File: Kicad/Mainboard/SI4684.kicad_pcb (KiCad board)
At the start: 2 copper layers, 100 x 68 mm, 91 parts, among them J1 DC IN, J2 Ant, J3 Headphones, J4 FRONT-PCB, J5 AUDIO, U1 MIC5504-1.8YM5, U2 LM2596T-5, U3 SI4684-A10-GM, U4 LM1117T-3.3, U5 TPA6130A2RTJTG4, U6 NE5532, X1 19.2MHz

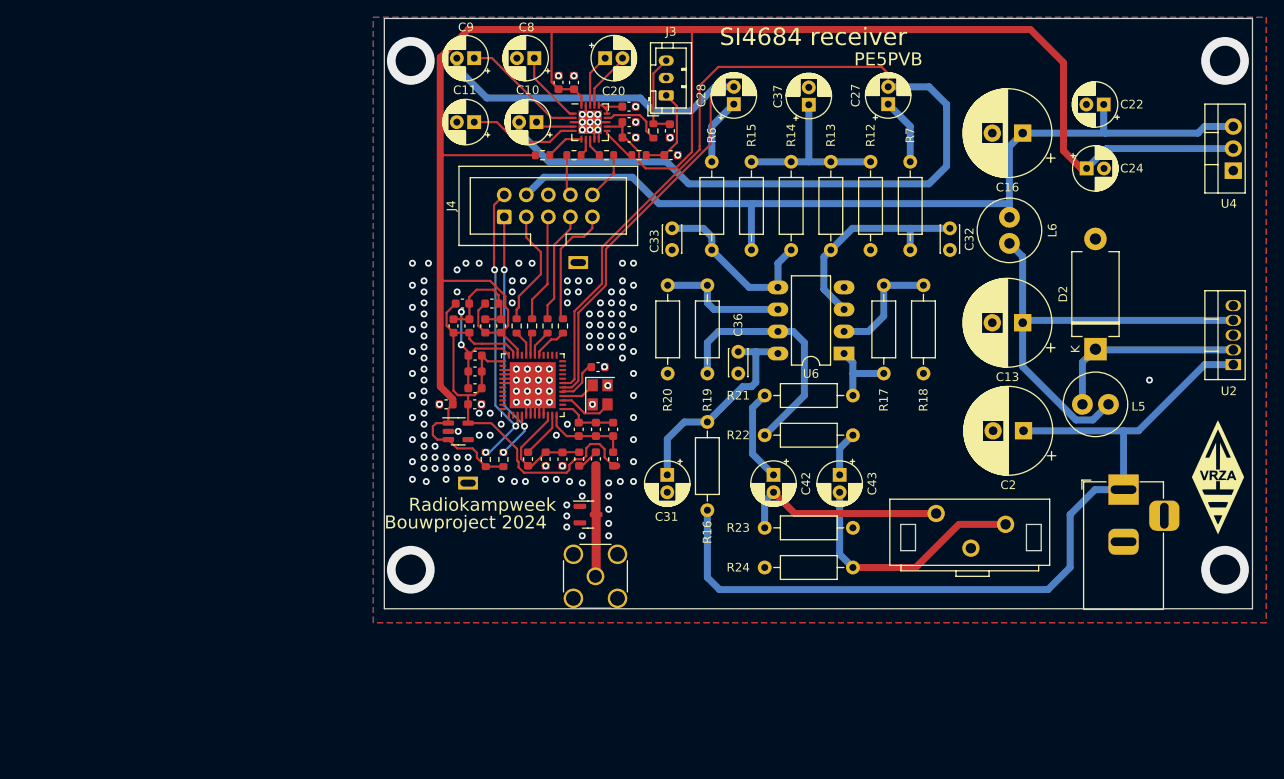
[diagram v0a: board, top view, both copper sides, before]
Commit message: Add files via upload
work in progress. not finished
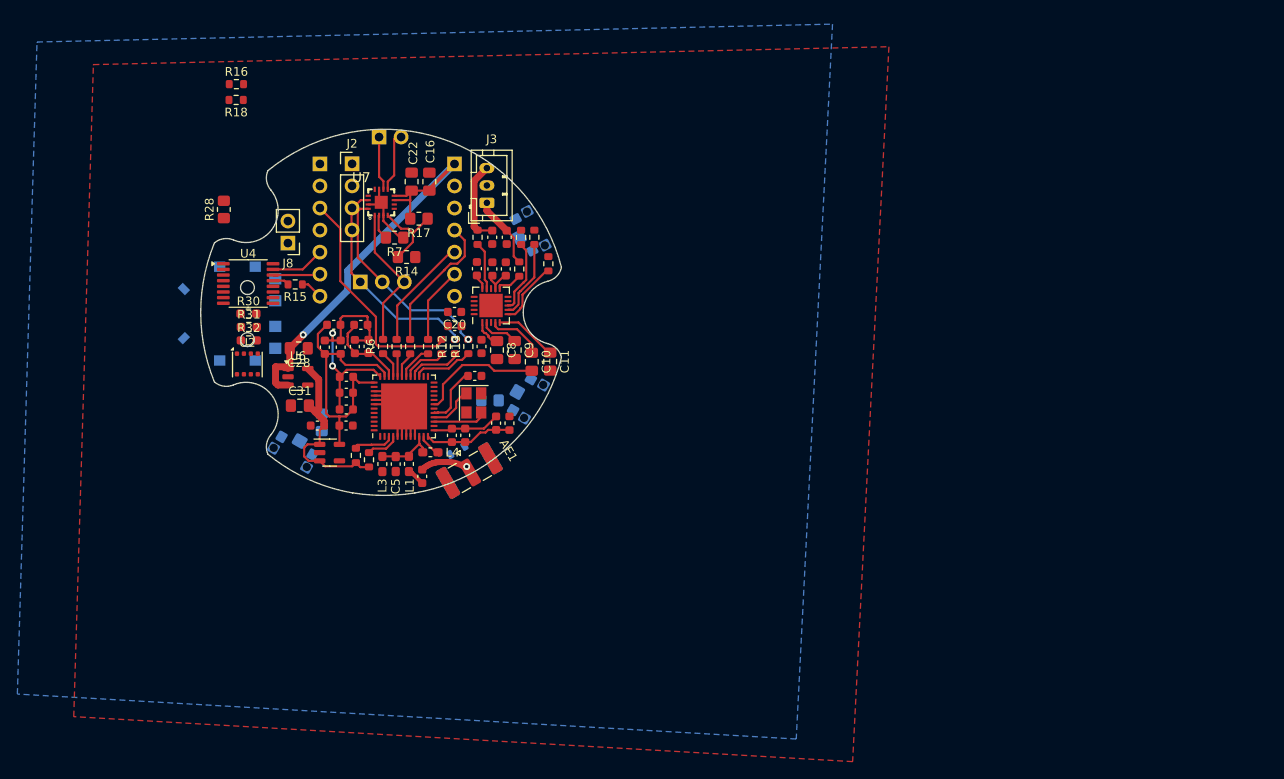
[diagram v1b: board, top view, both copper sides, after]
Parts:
- removed C13, C2: 220uF, Capacitor_THT:CP_Radial_D10.0mm_P3.50mm
- removed C24, C27, C37: 10uF, Capacitor_THT:CP_Radial_D5.0mm_P2.00mm
- removed C32, C33, C36: 10p, Capacitor_THT:C_Disc_D3.0mm_W2.0mm_P2.50mm
- removed C42, C43: 47uF, Capacitor_THT:CP_Radial_D5.0mm_P2.00mm
- removed D2: 1N5822, Diode_THT:D_DO-201_P12.70mm_Horizontal
- removed G***: LOGO, Library:VRZA
- removed J4: FRONT-PCB, Connector_IDC:IDC-Header_2x05_P2.54mm_Vertical
- removed L5: 33uH, Inductor_THT:L_Radial_D7.2mm_P3.00mm_Murata_1700
- removed L6: 22uH, Inductor_THT:L_Radial_D7.2mm_P3.00mm_Murata_1700
- removed R19: 4k7, Resistor_THT:R_Axial_DIN0207_L6.3mm_D2.5mm_P10.16mm_Horizontal
- removed R20: 3k9, Resistor_THT:R_Axial_DIN0207_L6.3mm_D2.5mm_P10.16mm_Horizontal
- removed R21, R22: 220, Resistor_THT:R_Axial_DIN0207_L6.3mm_D2.5mm_P10.16mm_Horizontal
- removed R23, R24: 100k, Resistor_THT:R_Axial_DIN0207_L6.3mm_D2.5mm_P10.16mm_Horizontal
- removed REF**: 25x25 can, Library:25x25 can
- added AE1: Antenna_Shield, Connector_Coaxial:SMA_Samtec_SMA-J-P-H-ST-EM1_EdgeMount, F.Cu at (109.5, 118.6)
- added J6: DISP RIGHT, Connector_PinHeader_2.54mm:PinHeader_1x07_P2.54mm_Vertical, B.Cu at (107.6, 83.0)
- added J7: Conn_01x02_Pin, Connector_PinHeader_2.54mm:PinHeader_1x02_P2.54mm_Vertical, B.Cu at (99.0, 80.0)
- added J8: Conn_01x02_Pin, Connector_PinHeader_2.54mm:PinHeader_1x02_P2.54mm_Vertical, F.Cu at (88.5, 92.2)
- added R27: 10k, Resistor_SMD:R_0805_2012Metric_Pad1.20x1.40mm_HandSolder, B.Cu at (92.4, 112.8)
- added R28: 10k, Resistor_SMD:R_0805_2012Metric_Pad1.20x1.40mm_HandSolder, F.Cu at (81.1, 88.3)
- added R29: 10k, Resistor_SMD:R_0805_2012Metric_Pad1.20x1.40mm_HandSolder, B.Cu at (111.7, 110.3)
- added R30: 10k, Resistor_SMD:R_0603_1608Metric_Pad0.98x0.95mm_HandSolder, F.Cu at (83.9, 100.3)
- added R31: 10k, Resistor_SMD:R_0603_1608Metric_Pad0.98x0.95mm_HandSolder, F.Cu at (84.0, 101.8)
- added R32: 10k, Resistor_SMD:R_0603_1608Metric_Pad0.98x0.95mm_HandSolder, F.Cu at (84.0, 103.4)
- added SW4: SW_Push, tp4056:SW_SPST_CK_KMS2xxGP, B.Cu at (89.1, 116.2)
- added SW5: SW_Push, tp4056:SW_SPST_CK_KMS2xxGP, B.Cu at (116.4, 90.8)
- added SW6: SW_Push, tp4056:SW_SPST_CK_KMS2xxGP, B.Cu at (116.1, 110.0)
- added U12: SIQ-02FVS3, tp4056:SW-SMD_SIQ-02FVS3_1, B.Cu at (81.7, 100.3)
- added U7: ~, tp4056:TQFN-16_L3.0-W3.0-P0.50-BL-EP1.5, F.Cu at (99.2, 87.5)
- C10, C28, C31, C9: value 10uF -> 1uF; footprint Capacitor_THT:CP_Radial_D5.0mm_P2.00mm -> Capacitor_SMD:C_0805_2012Metric_Pad1.18x1.45mm_HandSolder
- C11, C8: footprint Capacitor_THT:CP_Radial_D5.0mm_P2.00mm -> Capacitor_SMD:C_0805_2012Metric_Pad1.18x1.45mm_HandSolder
- C16: value 100uF -> 10uF; footprint Capacitor_THT:CP_Radial_D10.0mm_P3.50mm -> Capacitor_SMD:C_0805_2012Metric_Pad1.18x1.45mm_HandSolder
- C20: footprint Capacitor_THT:CP_Radial_D5.0mm_P2.00mm -> Capacitor_SMD:C_0603_1608Metric
- C22: value 10uF -> 100nF; footprint Capacitor_THT:CP_Radial_D5.0mm_P2.00mm -> Capacitor_SMD:C_0805_2012Metric_Pad1.18x1.45mm_HandSolder
- C5: footprint Capacitor_SMD:C_0603_1608Metric -> Capacitor_SMD:C_0603_1608Metric_Pad1.08x0.95mm_HandSolder
- D1: footprint Package_TO_SOT_SMD:SOT-23 -> Package_TO_SOT_SMD:SOT-23W; moved to B.Cu
- J1: value DC IN -> Conn_01x03; footprint Connector_BarrelJack:BarrelJack_Horizontal -> Connector_PinHeader_2.54mm:PinHeader_1x03_P2.54mm_Vertical; moved to B.Cu
- J2: value Ant -> Conn_01x04_Pin; footprint Connector_Coaxial:SMA_Amphenol_132134-16_Vertical -> Connector_PinHeader_2.54mm:PinHeader_1x04_P2.54mm_Vertical
- J5: value AUDIO -> DISP LEFT; footprint Library:FC68405_cinch -> Connector_PinHeader_2.54mm:PinHeader_1x07_P2.54mm_Vertical; moved to B.Cu
- L1, L3, L4: footprint Inductor_SMD:L_0603_1608Metric -> Inductor_SMD:L_0603_1608Metric_Pad1.05x0.95mm_HandSolder
- R12: value 39k -> 2k; footprint Resistor_THT:R_Axial_DIN0207_L6.3mm_D2.5mm_P10.16mm_Horizontal -> Resistor_SMD:R_0603_1608Metric
- R13: value 100k -> 2k; footprint Resistor_THT:R_Axial_DIN0207_L6.3mm_D2.5mm_P10.16mm_Horizontal -> Resistor_SMD:R_0603_1608Metric
- R14: value 100k -> 3k; footprint Resistor_THT:R_Axial_DIN0207_L6.3mm_D2.5mm_P10.16mm_Horizontal -> Resistor_SMD:R_0805_2012Metric_Pad1.20x1.40mm_HandSolder
- R15: value 39k -> 100; footprint Resistor_THT:R_Axial_DIN0207_L6.3mm_D2.5mm_P10.16mm_Horizontal -> Resistor_SMD:R_0603_1608Metric
- R16: value 10 -> 0; footprint Resistor_THT:R_Axial_DIN0207_L6.3mm_D2.5mm_P10.16mm_Horizontal -> Resistor_SMD:R_0603_1608Metric
- R17: value 4k7 -> 680K; footprint Resistor_THT:R_Axial_DIN0207_L6.3mm_D2.5mm_P10.16mm_Horizontal -> Resistor_SMD:R_0805_2012Metric_Pad1.20x1.40mm_HandSolder
- R18: value 3k9 -> 0; footprint Resistor_THT:R_Axial_DIN0207_L6.3mm_D2.5mm_P10.16mm_Horizontal -> Resistor_SMD:R_0603_1608Metric
- R6: value 4k7 -> 600; footprint Resistor_THT:R_Axial_DIN0207_L6.3mm_D2.5mm_P10.16mm_Horizontal -> Resistor_SMD:R_0603_1608Metric
- R7: value 4k7 -> 100K; footprint Resistor_THT:R_Axial_DIN0207_L6.3mm_D2.5mm_P10.16mm_Horizontal -> Resistor_SMD:R_0805_2012Metric_Pad1.20x1.40mm_HandSolder
- U2: value LM2596T-5 -> BME680; footprint Package_TO_SOT_THT:TO-220-5_Vertical -> Package_LGA:Bosch_LGA-8_3x3mm_P0.8mm_ClockwisePinNumbering
- U4: value LM1117T-3.3 -> TCA9554PW; footprint Package_TO_SOT_THT:TO-220-3_Vertical -> Package_SO:TSSOP-16_4.4x5mm_P0.65mm
- U6: value NE5532 -> RT9013; footprint Package_DIP:DIP-8_W7.62mm_LongPads -> Package_TO_SOT_SMD:SOT-23-5
- moved U4 114.2 mm to (83.9, 96.8), turned to 0 degrees
- moved U2 113.6 mm to (83.8, 106.1), turned to 0 degrees
- moved J1 91.1 mm to (96.8, 96.6), turned to -90 degrees
- moved J5 85.3 mm to (92.1, 83.0)
- moved R18 82.0 mm to (82.5, 75.7), turned to 180 degrees
- moved C22 80.2 mm to (102.7, 85.1), turned to 90 degrees
- moved R16 73.2 mm to (82.5, 73.9), turned to 0 degrees
- moved C16 68.6 mm to (104.8, 85.1), turned to 90 degrees
- moved U6 63.0 mm to (89.6, 107.6), turned to 0 degrees
- moved R7 60.0 mm to (100.8, 91.5), turned to 180 degrees
- moved C28 57.5 mm to (89.7, 104.3), turned to 180 degrees
- moved J2 55.2 mm to (95.8, 83.0)
- moved R15 54.4 mm to (89.3, 96.9), turned to 180 degrees
- moved R17 54.1 mm to (103.5, 89.4), turned to 180 degrees
- moved R12 49.1 mm to (107.7, 104.1)
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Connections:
- C28 pad 1: Net-(C28-Pad1) -> GND
- C28 pad 2: L -> +5V
- C3 pad 1: Net-(J2-In) -> Net-(AE1-A)
- C31 pad 1: Net-(U6C-V+) -> GND
- C31 pad 2: GND -> +3V3
- D1 pad 3: Net-(J2-In) -> Net-(AE1-A)
- J1 pad 1: +12V -> I2SLRC
- J1 pad 2: GND -> I2SCLK
- J1 pad 3: GND -> I2SDIN
- J2 pad 1: Net-(J2-In) -> A
- J2 pad 2: GND -> B
- J5 pad 1: Net-(J5-IN1) -> RST
- J5 pad 2: Net-(J5-IN2) -> LCD_CS
- J5 pad 3: GND -> SS
- R12 pad 1: GND -> Net-(U3-DSF)
- R12 pad 2: Net-(C37-Pad1) -> I2SLRC
- R13 pad 1: Net-(U6A-+) -> Net-(U3-DCLK)
- R13 pad 2: Net-(C37-Pad1) -> I2SCLK
- R14 pad 1: Net-(C37-Pad1) -> I2SD
- R14 pad 2: Net-(U6B-+) -> Net-(U7-SD)
- R15 pad 1: Net-(C37-Pad1) -> INT
- R15 pad 2: +5V -> Net-(U4-~{INT})
- R16 pad 1: +12V -> +3V3
- R16 pad 2: Net-(U6C-V+) -> A
- R17 pad 1: Net-(U6A--) -> Net-(U7-SD)
- R17 pad 2: Net-(R17-Pad2) -> +5V
- R18 pad 1: Net-(U6A--) -> GND
- R18 pad 2: GND -> B
- R6 pad 1: Net-(C28-Pad1) -> Net-(U3-DOUT)
- R6 pad 2: Net-(U6B-+) -> I2SDIN
- R7 pad 1: Net-(C27-Pad1) -> GND
- R7 pad 2: Net-(U6A-+) -> Net-(U7-GAIN)
- U2 pad 1: +12V -> unconnected-(U2-GND-Pad1)
- U2 pad 2: Net-(D2-K) -> unconnected-(U2-CSB-Pad2)
- U2 pad 3: GND -> unconnected-(U2-SDI-Pad3)
- U2 pad 4: Net-(U2-FB) -> unconnected-(U2-SCK-Pad4)
- U2 pad 5: GND -> unconnected-(U2-SDO-Pad5)
- U3 pad 27: unconnected-(U3-DCLK-Pad27) -> Net-(U3-DCLK)
- U3 pad 28: unconnected-(U3-DSF-Pad28) -> Net-(U3-DSF)
- U3 pad 33: unconnected-(U3-DOUT-Pad33) -> Net-(U3-DOUT)
- U4 pad 2: +3V3 -> GND
- U4 pad 3: +5V -> GND
- U6 pad 1: Net-(R17-Pad2) -> +5V
- U6 pad 2: Net-(U6A--) -> GND
- U6 pad 3: Net-(U6A-+) -> +5V
- U6 pad 4: GND -> unconnected-(U6-FB-Pad4)
- U6 pad 5: Net-(U6B-+) -> +3V3
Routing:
- net +3V3: track 235.6 -> 35.5 mm
- net R: track 134.2 -> 14.5 mm
- net +12V: track 98.7 -> 0.00 mm
- net L: track 80.8 -> 0.00 mm
- net Net-(U2-FB): track 52.4 -> 0.00 mm
- net +5V: track 101.4 -> 49.9 mm, vias 0 -> 1
- net Net-(J5-IN2): track 29.0 -> 0.00 mm
- net Net-(R19-Pad2): track 28.4 -> 0.00 mm
- net INT: track 34.2 -> 7.36 mm, vias 3 -> 0
- net RST: track 30.5 -> 3.91 mm, vias 3 -> 0
- net Net-(U6A-+): track 25.4 -> 0.00 mm
- net Net-(U6C-V+): track 25.2 -> 0.00 mm
- net I2SLRC: track 0.00 -> 25.1 mm, vias 0 -> 1
- net +1V8: track 57.6 -> 32.7 mm
- net Net-(J5-IN1): track 24.3 -> 0.00 mm
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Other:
- board size 100 x 68 mm -> 41.6 x 42.2 mm
- board text removed: "Bouwproject 2024"
- board text removed: "PE5PVB"
- board text removed: "Radiokampweek"
- board text removed: "SI4684 receiver"
